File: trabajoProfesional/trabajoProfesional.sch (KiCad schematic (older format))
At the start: 4 parts

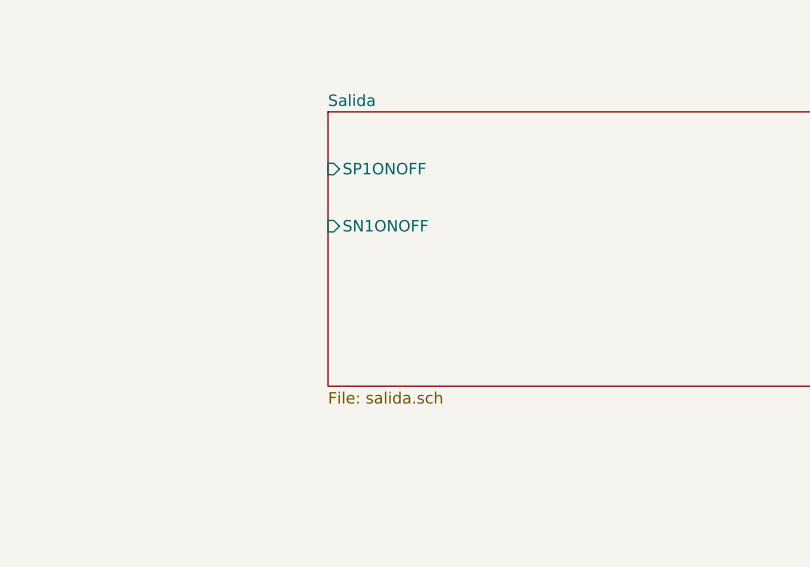
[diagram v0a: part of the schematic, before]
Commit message: ya tenemos los componentes falta el micro
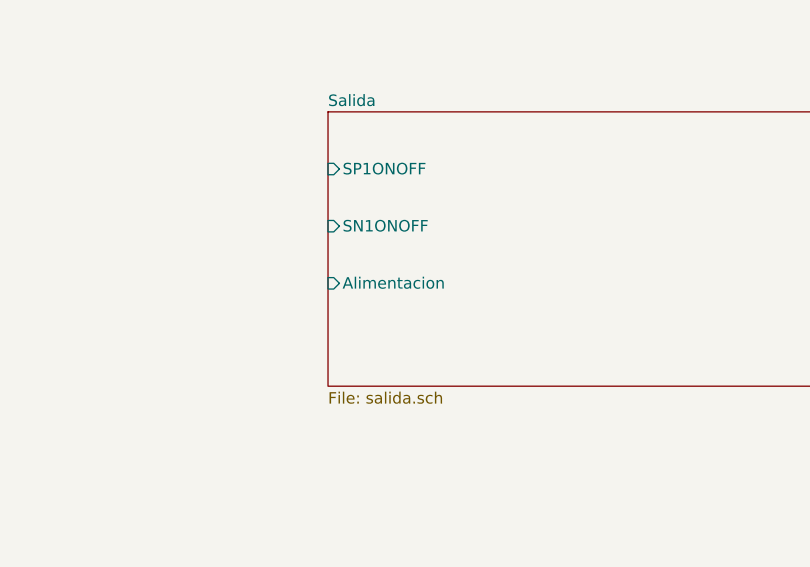
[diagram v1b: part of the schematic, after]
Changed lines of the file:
@@
 F2 "SP1ONOFF" I L 7950 2000 50
 F3 "SN1ONOFF" I L 7950 2250 50
+F4 "Alimentacion" I L 7950 2500 50
 $EndSheet
 $Comp
